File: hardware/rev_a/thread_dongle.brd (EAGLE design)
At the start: 20.9 x 14 mm, 24 parts, among them J1 USB-A-MALE-PLUG, J2 TC2030-JLINK-NL, U1 KW21Z, U2 ESDR0502N, U3 CP2102N-20, X1 FA-128, X2 FA-135

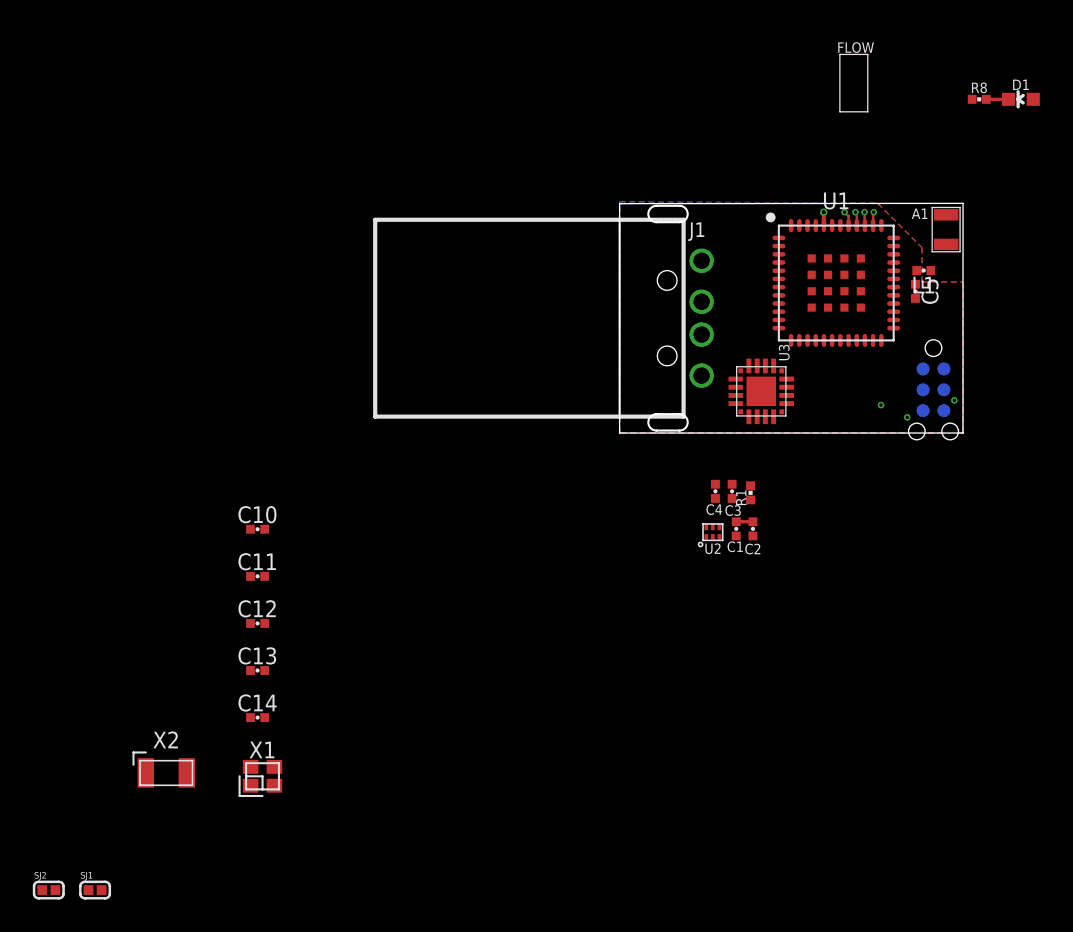
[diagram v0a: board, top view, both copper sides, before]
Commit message: Nothing to do and no errors
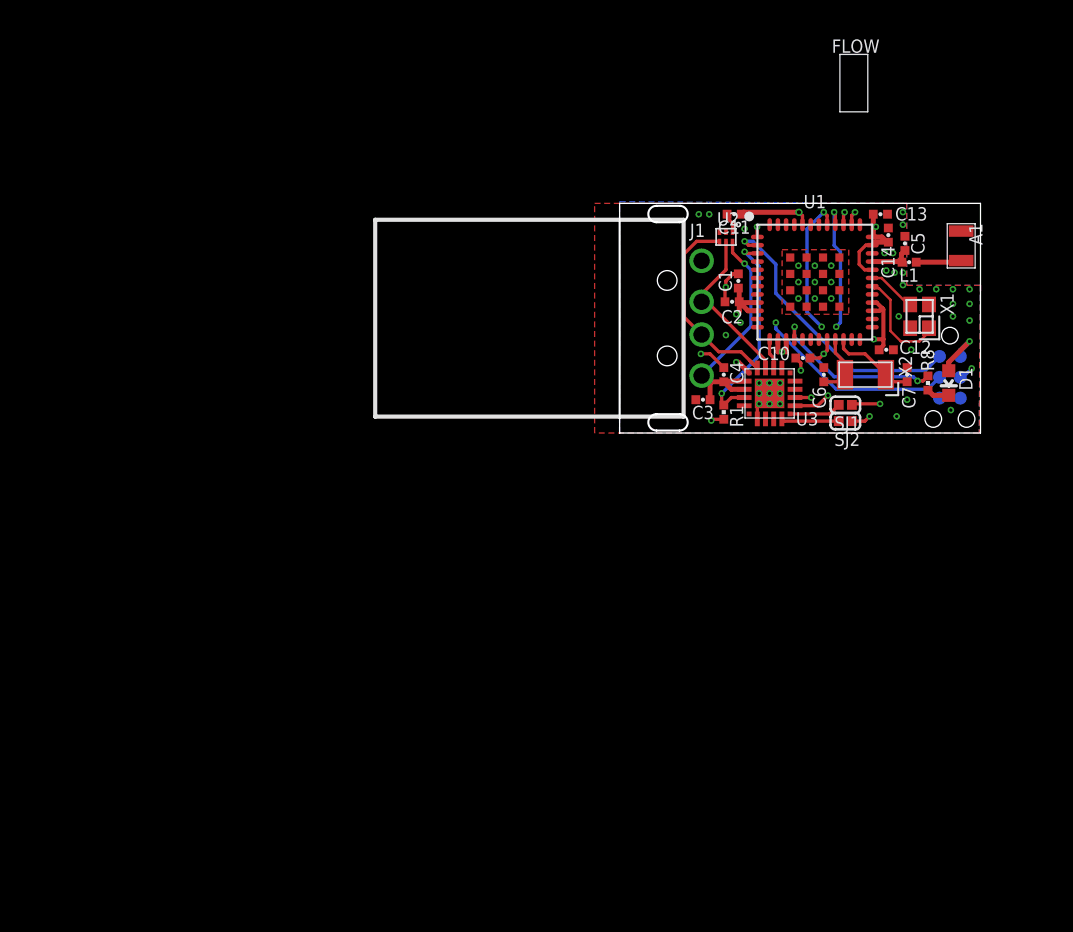
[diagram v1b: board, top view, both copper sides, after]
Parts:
- added C6, C7: 12pF, passives:0402_CAP
- moved SJ2 56.3 mm to (13.8, 0.72), turned to 180 degrees
- moved SJ1 54.5 mm to (13.8, 1.71), turned to 180 degrees
- moved X2 49.1 mm to (15.0, 3.56), turned to 180 degrees
- moved X1 48.9 mm to (18.3, 7.11), turned to 90 degrees
- moved C14 48.4 mm to (16.4, 12.1), turned to 90 degrees
- moved C13 47.1 mm to (15.9, 13.3)
- moved C12 41.8 mm to (16.3, 5.08)
- moved C11 36.5 mm to (6.99, 13.3), turned to 180 degrees
- moved C10 34.8 mm to (11.2, 4.57), turned to 180 degrees
- moved U2 18.0 mm to (6.49, 12.0), turned to 270 degrees
- moved D1 17.8 mm to (20.1, 3.05), turned to 180 degrees
- moved R8 17.6 mm to (18.8, 3.05), turned to 270 degrees
- moved C1 15.1 mm to (7.24, 9.27), turned to 90 degrees
- moved C2 13.9 mm to (6.86, 8.00), turned to 180 degrees
- moved C4 7.13 mm to (6.35, 3.56), turned to 90 degrees
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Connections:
- removed net N$11: U1.30, X1.3
- removed net N$14: U1.22, X2.1
- removed net N$15: U1.21, X2.2
- new net N$1: C6.1, U1.21, X2.2
- new net N$2: C7.1, U1.22, X2.1
- new net N$3: U1.31, X1.3
- net GND: now also C6.2, C7.2
- net N$12: now also U1.30; no longer U1.31
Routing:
- net !RESET: track 0.00 -> 31.3 mm, vias 0 -> 3
- net VCC: track 1.94 -> 29.0 mm, vias 1 -> 9
- net SWCLK: track 0.00 -> 19.1 mm, vias 0 -> 2
- net SWDIO: track 0.00 -> 17.4 mm, vias 0 -> 1
- net KW21Z_RTS: track 0.92 -> 16.5 mm, vias 1 -> 3
- net 5V: track 0.00 -> 15.2 mm, vias 0 -> 1
- net KW21Z_RX: track 0.83 -> 15.6 mm, vias 1 -> 2
- net KW21Z_CTS: track 0.85 -> 15.6 mm, vias 1 -> 3
- net KW21Z_TX: track 0.83 -> 14.7 mm, vias 1 -> 2
- net D-: track 0.00 -> 12.8 mm
- net N$8: track 0.08 -> 10.8 mm, vias 0 -> 2
- net D+: track 0.00 -> 10.1 mm
- net GND: track 0.00 -> 8.87 mm, vias 3 -> 47
- net N$12: track 0.00 -> 6.43 mm
- net N$2: track 0.00 -> 5.27 mm
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- added copper zone on layer 15, net VCC
- removed copper zone on layer 15, net GND
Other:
- board size 20.9 x 14 mm -> 22 x 14 mm
